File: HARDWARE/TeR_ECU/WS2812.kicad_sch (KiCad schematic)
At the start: 4 parts

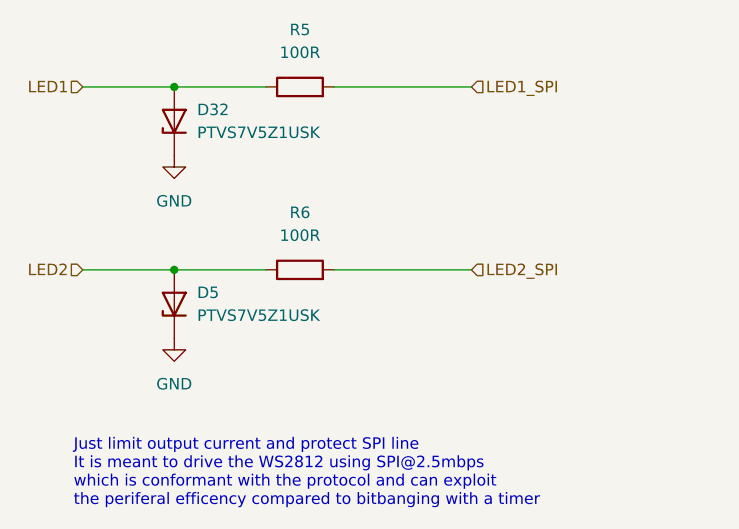
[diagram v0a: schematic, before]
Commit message: Finished layout, RF design, and quick DRC check, Lookin gud
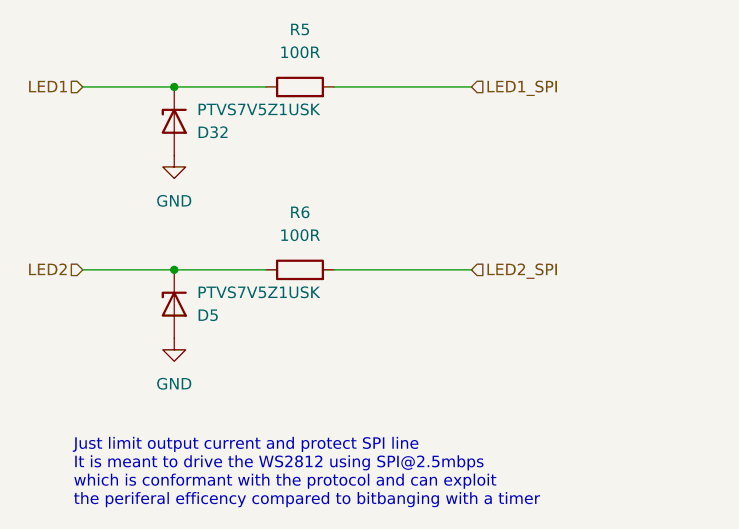
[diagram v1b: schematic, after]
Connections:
- net GND: now also D32.2 (A), D5.2 (A); no longer D32.1 (K), D5.1 (K)
- net LED1: now also D32.1 (K); no longer D32.2 (A)
- net LED2: now also D5.1 (K); no longer D5.2 (A)
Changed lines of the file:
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@@
 		(lib_id "Diode:PTVS7V5Z1USK")
 		(at 130.81 91.44 90)
+		(mirror x)
 		(unit 1)
 		(exclude_from_sim no)
@@
 		(on_board yes)
 		(dnp no)
-		(fields_autoplaced yes)
 		(property "Reference" "D5"
-			(at 133.35 90.1699 90)
+			(at 133.35 92.7101 90)
 			(effects
 				(font
@@
 		)
 		(property "Value" "PTVS7V5Z1USK"
-			(at 133.35 92.7099 90)
+			(at 133.35 90.1701 90)
 			(effects
 				(font
@@
 		(lib_id "Diode:PTVS7V5Z1USK")
 		(at 130.81 71.12 90)
+		(mirror x)
 		(unit 1)
 		(exclude_from_sim no)
@@
 		(on_board yes)
 		(dnp no)
-		(fields_autoplaced yes)
 		(property "Reference" "D32"
-			(at 133.35 69.8499 90)
+			(at 133.35 72.3901 90)
 			(effects
 				(font
@@
 		)
 		(property "Value" "PTVS7V5Z1USK"
-			(at 133.35 72.3899 90)
+			(at 133.35 69.8501 90)
 			(effects
 				(font
